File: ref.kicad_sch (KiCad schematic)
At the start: 14 parts, among them Q1 Q_NPN_BCE, U4 ADR1000, U5 Opamp_Dual

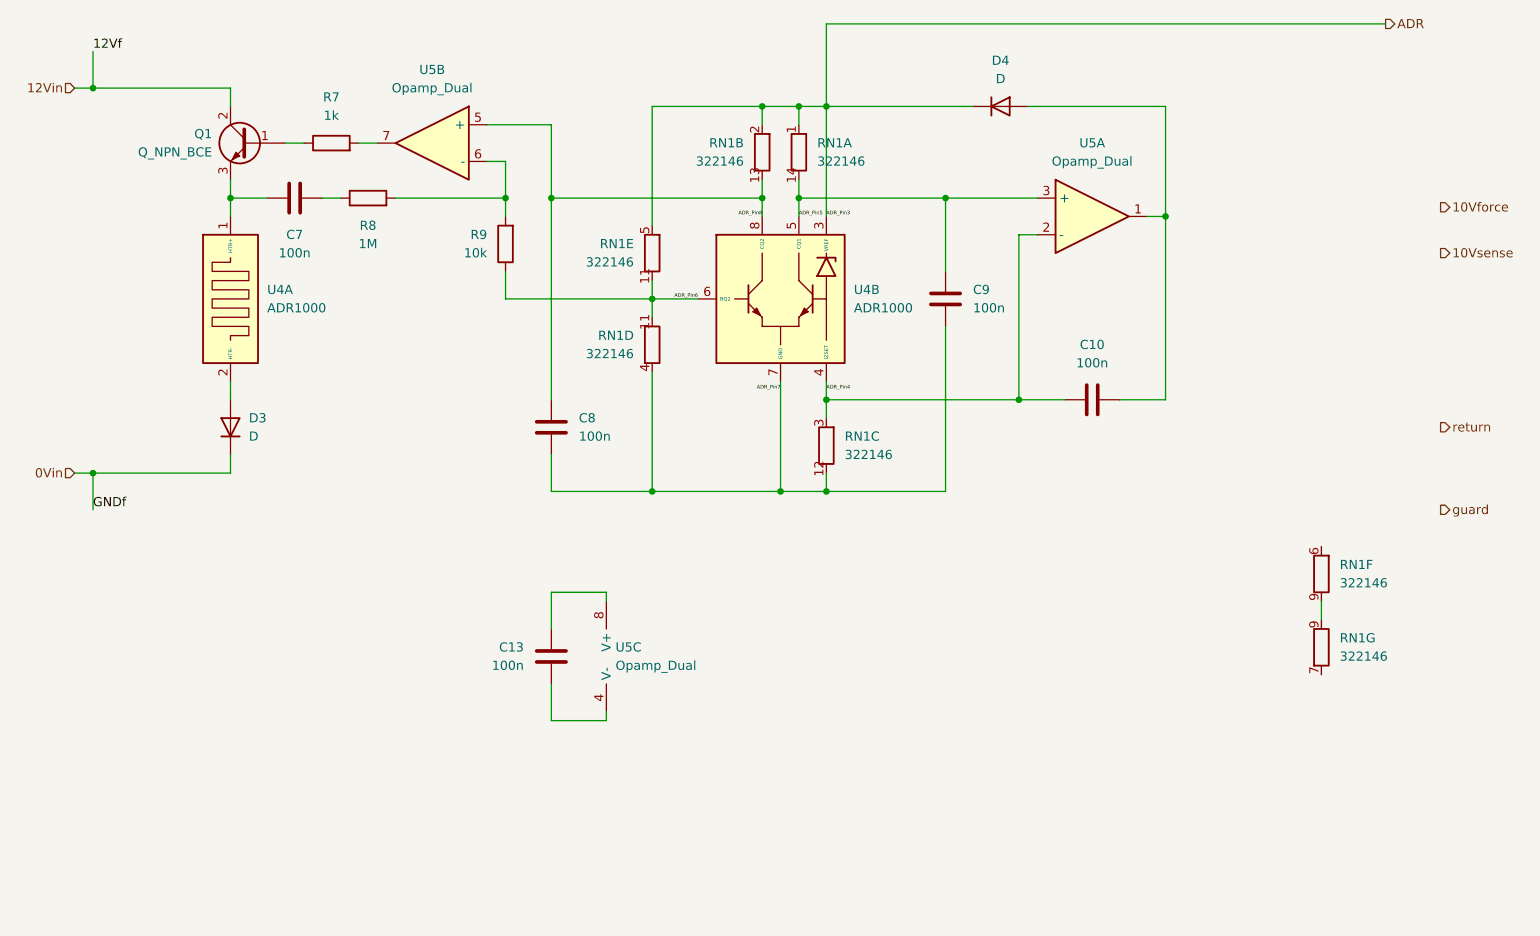
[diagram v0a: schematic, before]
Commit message: asas
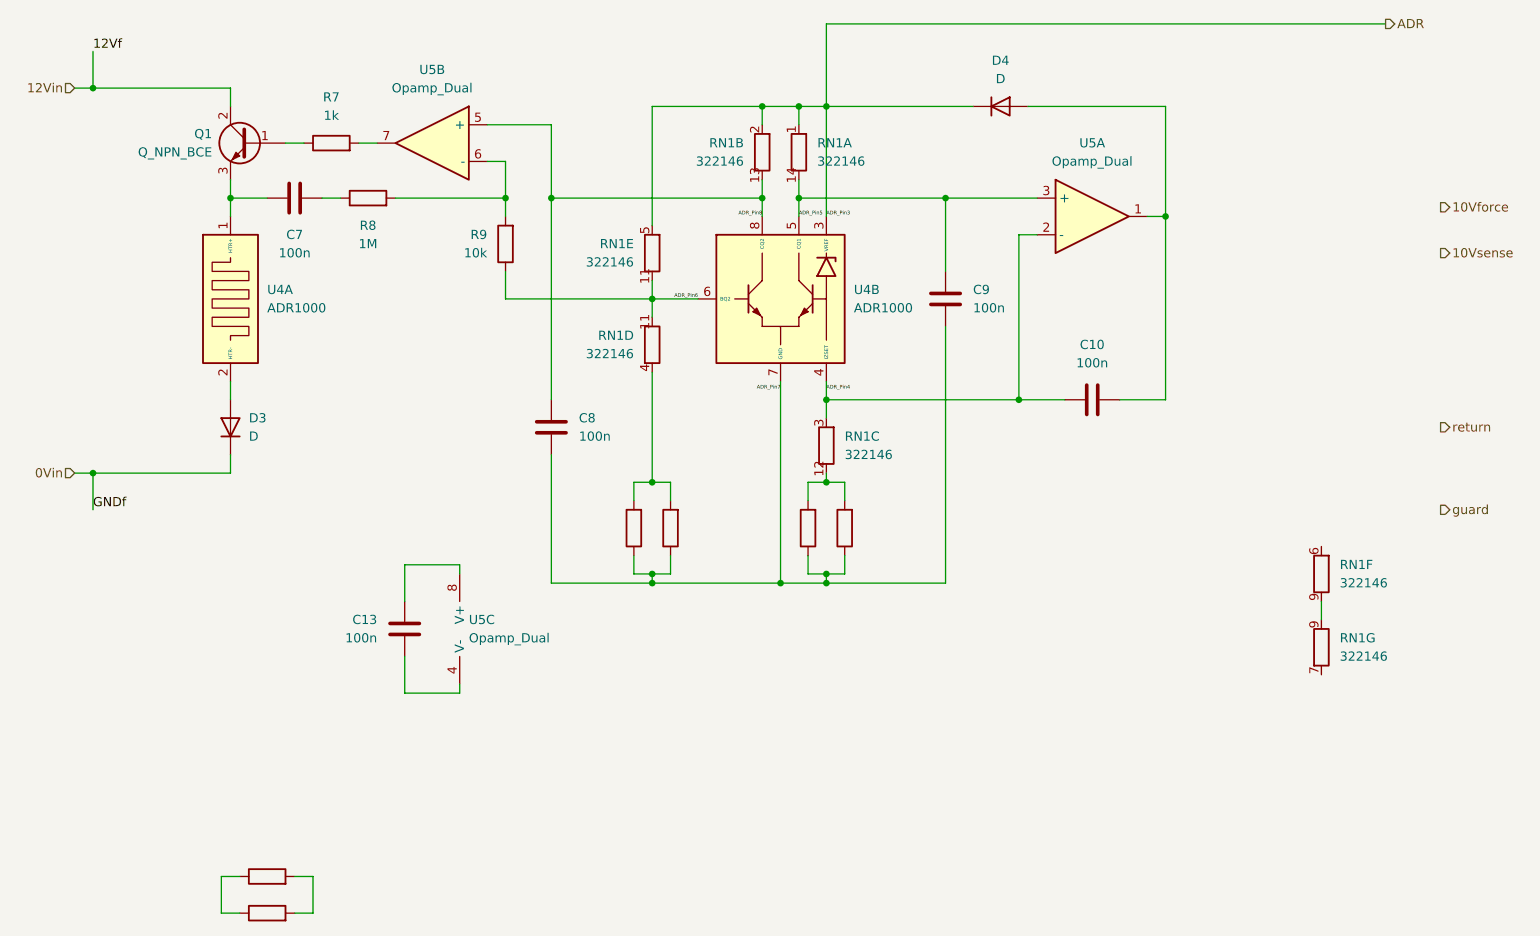
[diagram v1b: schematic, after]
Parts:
- added R13: dnp, Resistor_SMD:R_0805_2012Metric, symbol Device:R
- added R14: dnp, Crystal:Crystal_HC52-U_Vertical, symbol Device:R
- added R15, R17: 0, Resistor_SMD:R_0805_2012Metric, symbol Device:R
- added R16, R18: 0, Crystal:Crystal_HC52-U_Vertical, symbol Device:R
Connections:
- net ADR_Pin7: now also R15.1, R16.1, R17.1, R18.1; no longer RN1.12 (R3.2), RN1.4 (R4.1)
- new net: R17.2, R18.2, RN1.12 (R3.2)
- new net: R15.2, R16.2, RN1.4 (R4.1)
- new net: R13.1, R14.1
- new net: R13.2, R14.2
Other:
- moved on the sheet: C13, U5C
